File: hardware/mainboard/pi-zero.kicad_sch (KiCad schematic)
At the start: 48 parts, among them J24 Conn_01x05_Pin, J25 FPC 8p 0.5mm, J26 USB_A_Stacked, J27 USB_A_Stacked, T1 5V, T1 5VDet, T1 CS, T1 D+, T1 D-, T1 Gnd, T1 MISO, T1 MOSI, T1 RXD, T1 SClk, T1 Shield, T1 TXD, T1 V_{CC}, U13 USB2 Hub, Y2 12MHz

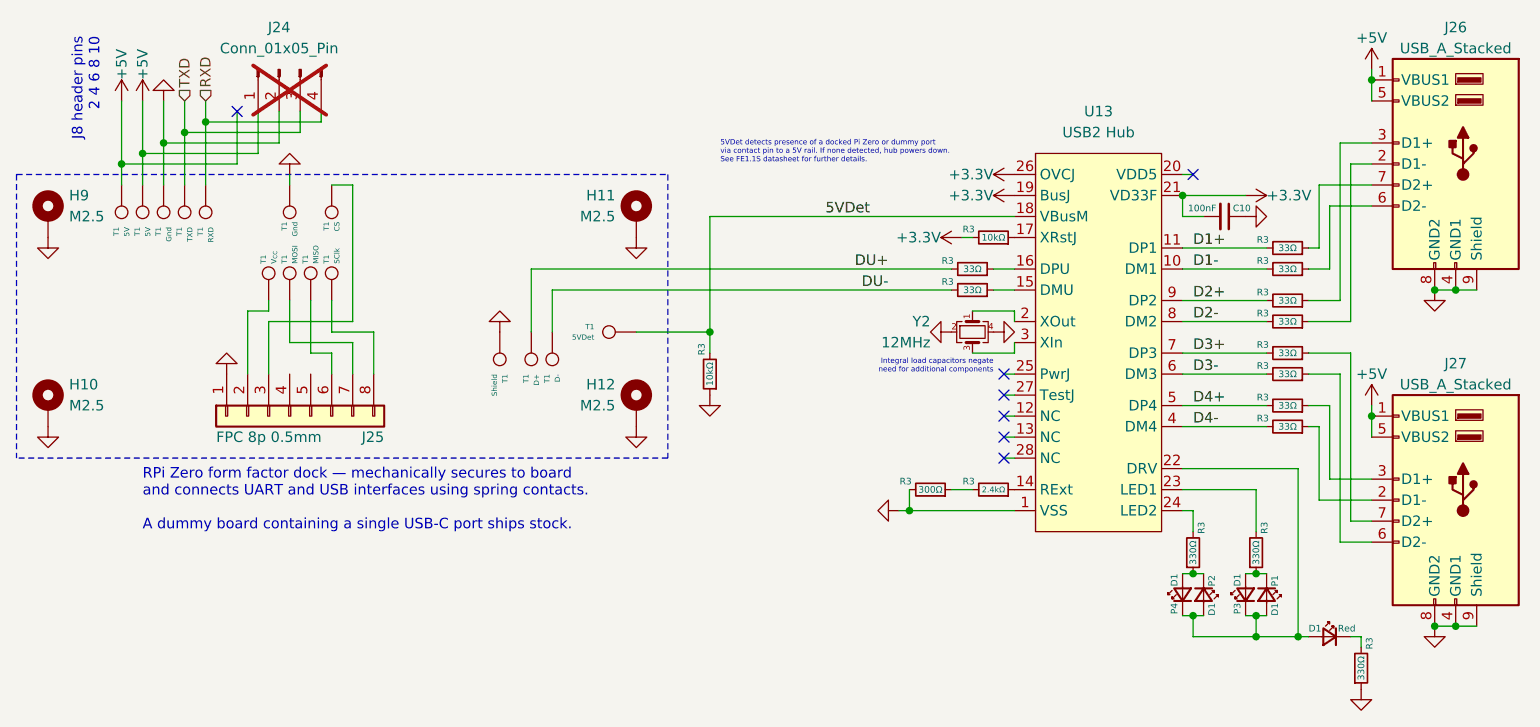
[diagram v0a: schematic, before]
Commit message: v0.2 feature complete
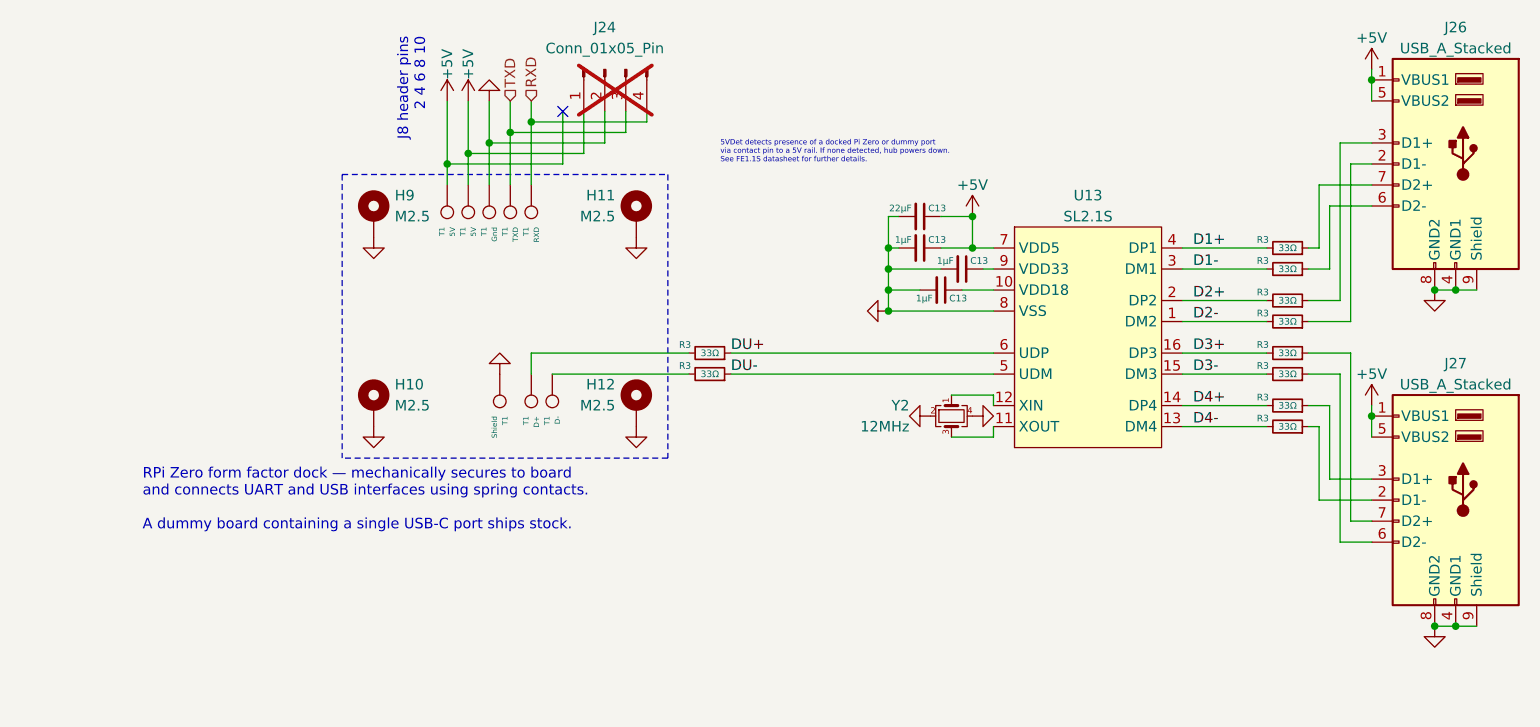
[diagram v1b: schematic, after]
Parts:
- removed C10: 100nF, AlphaLib:0402C, symbol Device:C_Small
- removed D1: P4, AlphaLib:0603LED, symbol Device:LED_Small
- removed D1: Red, AlphaLib:0603LED, symbol Device:LED_Small
- removed D1: P2, AlphaLib:0603LED, symbol Device:LED_Small
- removed D1: P3, AlphaLib:0603LED, symbol Device:LED_Small
- removed D1: P1, AlphaLib:0603LED, symbol Device:LED_Small
- removed J25: FPC 8p 0.5mm, Connector_FFC-FPC:Hirose_FH12-8S-0.5SH_1x08-1MP_P0.50mm_Horizontal, symbol Connector_Generic:Conn_01x08
- removed R3 (x3): 330Ω, AlphaLib:0402R, symbol Device:R_Small
- removed R3 (x2): 10kΩ, AlphaLib:0402R, symbol Device:R_Small
- removed R3: 300Ω, AlphaLib:0402R, symbol Device:R_Small
- removed R3: 2.4kΩ, AlphaLib:0402R, symbol Device:R_Small
- removed T1: Gnd, corevus:LGA_Spring_3.5x1, symbol Connector:TestPoint
- removed T1: MOSI, corevus:LGA_Spring_3.5x1, symbol Connector:TestPoint
- removed T1: V_{CC}, corevus:LGA_Spring_3.5x1, symbol Connector:TestPoint
- removed T1: 5VDet, corevus:LGA_Spring_3.5x1, symbol Connector:TestPoint
- removed T1: MISO, corevus:LGA_Spring_3.5x1, symbol Connector:TestPoint
- removed T1: CS, corevus:LGA_Spring_3.5x1, symbol Connector:TestPoint
- removed T1: SClk, corevus:LGA_Spring_3.5x1, symbol Connector:TestPoint
- removed U13: USB2 Hub, Package_SO:SSOP-28_3.9x9.9mm_P0.635mm, symbol corevus:FE1.1s-BSOP28B
- added C13 (x3): 1μF, AlphaLib:0402C, symbol Device:C_Small
- added C13: 22μF, Capacitor_SMD:C_1206_3216Metric, symbol Device:C_Small
- added U13: SL2.1S, corevus:SL2.1S, symbol corevus:SL2.1S
- T1: footprint corevus:LGA_Spring_3.5x1 -> corevus:LGA_Spring
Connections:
- net +5V: now also C13.1, C13.1, U13.7 (VDD5)
- net D1+: now also U13.4 (DP1)
- net D1-: now also U13.3 (DM1)
- net D2+: now also U13.2 (DP2)
- net D2-: now also U13.1 (DM2)
- net D3+: now also U13.16 (DP3)
- net D3-: now also U13.15 (DM3)
- net D4+: now also U13.14 (DP4)
- net D4-: now also U13.13 (DM4)
- net DU+: now also R3.1, U13.6 (UDP); no longer R3.2, T1.1
- net DU-: now also R3.1, U13.5 (UDM); no longer R3.2, T1.1
- net GND: now also C13.2, C13.2, C13.2, C13.2, U13.8 (VSS)
- net at Y2.1: now also U13.12 (XIN)
- net at Y2.3: now also U13.11 (XOUT)
- new net: C13.1, U13.9 (VDD33)
- new net: R3.2, T1.1 (x2)
- new net: C13.1, U13.10 (VDD18)
- no-connect marks 7 -> 1
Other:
- note removed: "Integral load capacitors negate need for additional components"
- moved on the sheet: H10, H9, J24, R3, T1, Y2
